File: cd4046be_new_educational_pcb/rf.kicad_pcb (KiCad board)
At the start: 2 copper layers, 84.5 x 60.5 mm, 36 parts, among them IC1 CD4046BE, J1 Conn_01x02_Socket, J2 Conn_01x08_Socket, J3 Conn_01x08_Socket, J4 Conn_01x02_Socket, J5 Conn_01x02_Socket, J6 Conn_01x02_Socket, J7 Conn_01x02_Socket, J8 Conn_01x02_Socket

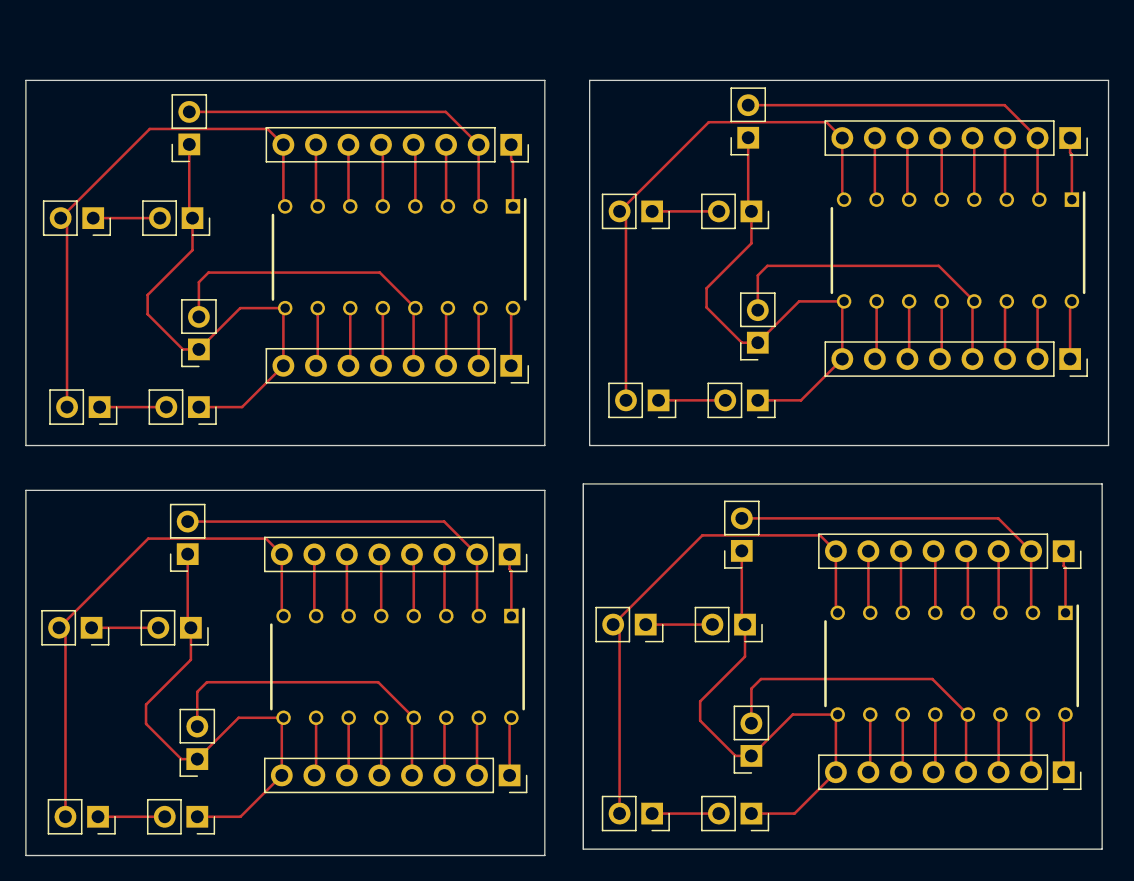
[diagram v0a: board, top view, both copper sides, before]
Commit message: α
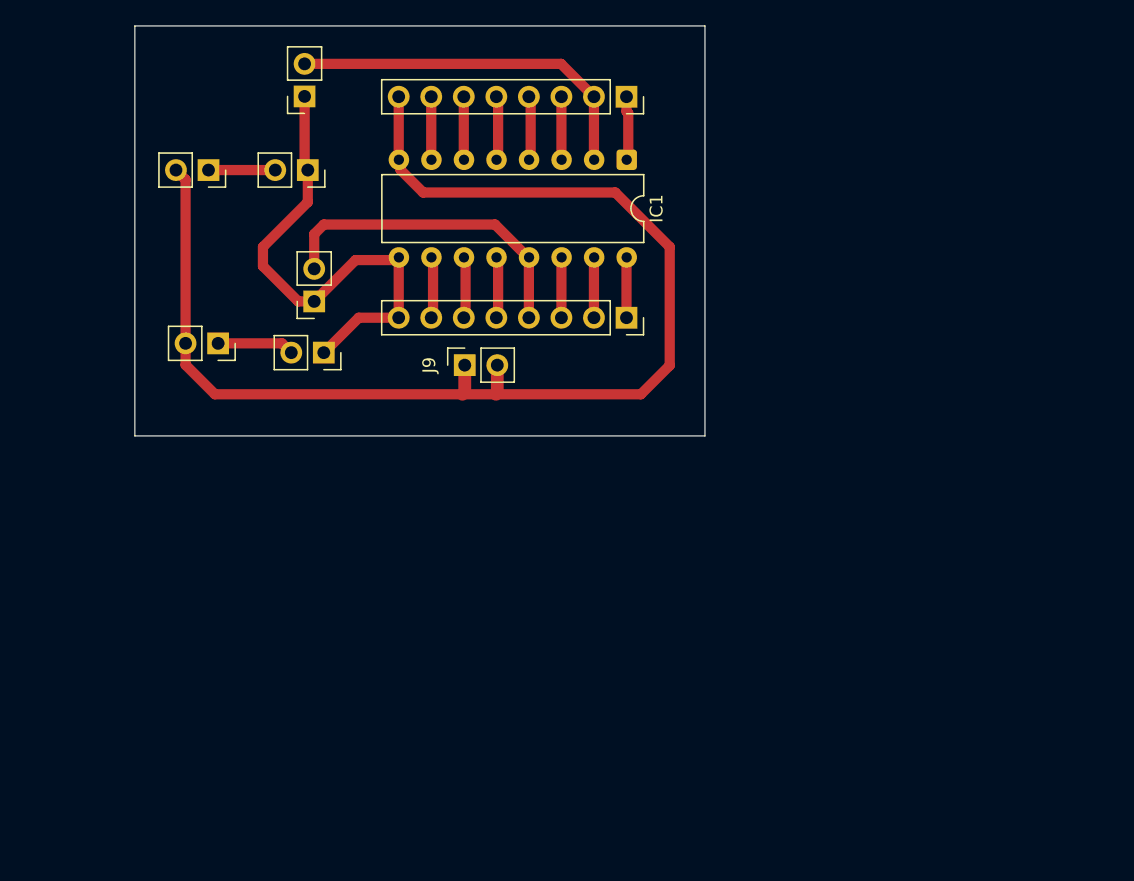
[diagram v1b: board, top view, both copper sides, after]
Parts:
- removed the IC1 at (154.0, 127.0)
- removed the IC1 at (197.8, 94.5)
- removed the IC1 at (197.2, 126.8)
- removed the IC1 at (154.1, 95.1)
- removed the J1 at (137.6, 118.2)
- removed the J1 at (180.9, 118.0)
- removed the J1 at (181.4, 85.7)
- removed the J1 at (137.8, 86.2)
- removed the J2 at (162.8, 118.2)
- removed the J2 at (162.9, 86.3)
- removed the J2 at (206.0, 118.0)
- removed the J2 at (206.5, 85.8)
- removed the J3 at (162.8, 135.5)
- removed the J3 at (206.0, 135.2)
- removed the J3 at (162.9, 103.5)
- removed the J3 at (206.5, 103.0)
- removed the J4 at (181.1, 123.7)
- removed the J4 at (137.9, 124.0)
- removed the J4 at (181.6, 91.5)
- removed the J4 at (138.0, 92.0)
- removed the J5 at (130.2, 92.0)
- removed the J5 at (130.1, 124.0)
- removed the J5 at (173.4, 123.7)
- removed the J5 at (173.9, 91.5)
- removed the J6 at (182.1, 101.7)
- removed the J6 at (181.6, 134.0)
- removed the J6 at (138.4, 134.2)
- removed the J6 at (138.5, 102.2)
- removed the J7 at (130.6, 138.7)
- removed the J7 at (130.8, 106.8)
- removed the J7 at (173.9, 138.5)
- removed the J7 at (174.4, 106.2)
- removed the J8 at (138.4, 138.7)
- removed the J8 at (182.1, 106.2)
- removed the J8 at (181.6, 138.5)
- removed the J8 at (138.5, 106.8)
- added IC1: CD4046BE, Package_DIP:CERDIP-16_W7.62mm_SideBrazed, F.Cu at (171.9, 87.4)
- added J1: Conn_01x02_Socket, Connector_PinSocket_2.54mm:PinSocket_1x02_P2.54mm_Vertical, F.Cu at (146.8, 82.5)
- added J2: Conn_01x08_Socket, Connector_PinSocket_2.54mm:PinSocket_1x08_P2.54mm_Vertical, F.Cu at (171.9, 82.5)
- added J3: Conn_01x08_Socket, Connector_PinSocket_2.54mm:PinSocket_1x08_P2.54mm_Vertical, F.Cu at (171.9, 99.8)
- added J4: Conn_01x02_Socket, Connector_PinSocket_2.54mm:PinSocket_1x02_P2.54mm_Vertical, F.Cu at (147.0, 88.2)
- added J5: Conn_01x02_Socket, Connector_PinSocket_2.54mm:PinSocket_1x02_P2.54mm_Vertical, F.Cu at (139.2, 88.2)
- added J6: Conn_01x02_Socket, Connector_PinSocket_2.54mm:PinSocket_1x02_P2.54mm_Vertical, F.Cu at (147.5, 98.5)
- added J7: Conn_01x02_Socket, Connector_PinSocket_2.54mm:PinSocket_1x02_P2.54mm_Vertical, F.Cu at (140.0, 101.8)
- added J8: Conn_01x02_Socket, Connector_PinSocket_2.54mm:PinSocket_1x02_P2.54mm_Vertical, F.Cu at (148.2, 102.5)
- added J9: Conn_01x02_Socket, Connector_PinSocket_2.54mm:PinSocket_1x02_P2.54mm_Vertical, F.Cu at (159.2, 103.5)
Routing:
- net /VCO_IN: track 166.6 -> 40.7 mm
- net /PC1: track 114.1 -> 28.5 mm
- net /PC2: track 102.5 -> 25.6 mm
- net GND: track 162.4 -> 98.4 mm
- net Net-(J4-Pin_2): track 20.8 -> 5.21 mm
- net Net-(J7-Pin_1): track 20.8 -> 6.01 mm
- net Net-(IC1-VCO_OUT): track 19.5 -> 4.87 mm
- net Net-(IC1-COMPARATOR_IN): track 19.5 -> 4.87 mm
- net Net-(IC1-CI(2)): track 19.5 -> 4.87 mm
- net Net-(IC1-PHASE_PULSES): track 19.5 -> 4.87 mm
- net Net-(IC1-INHIBIT): track 19.5 -> 4.87 mm
- net Net-(IC1-CI(1)): track 19.5 -> 4.87 mm
- net Net-(IC1-SIGNAL_IN): track 18.2 -> 4.56 mm
- net Net-(IC1-DEMODULATOR_OUT): track 18.2 -> 4.56 mm
- net VDD: track 18.2 -> 4.56 mm
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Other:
- board size 84.5 x 60.5 mm -> 44.5 x 32 mm
